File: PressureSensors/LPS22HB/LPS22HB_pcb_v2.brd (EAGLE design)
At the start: 100 x 80 mm, 6 parts

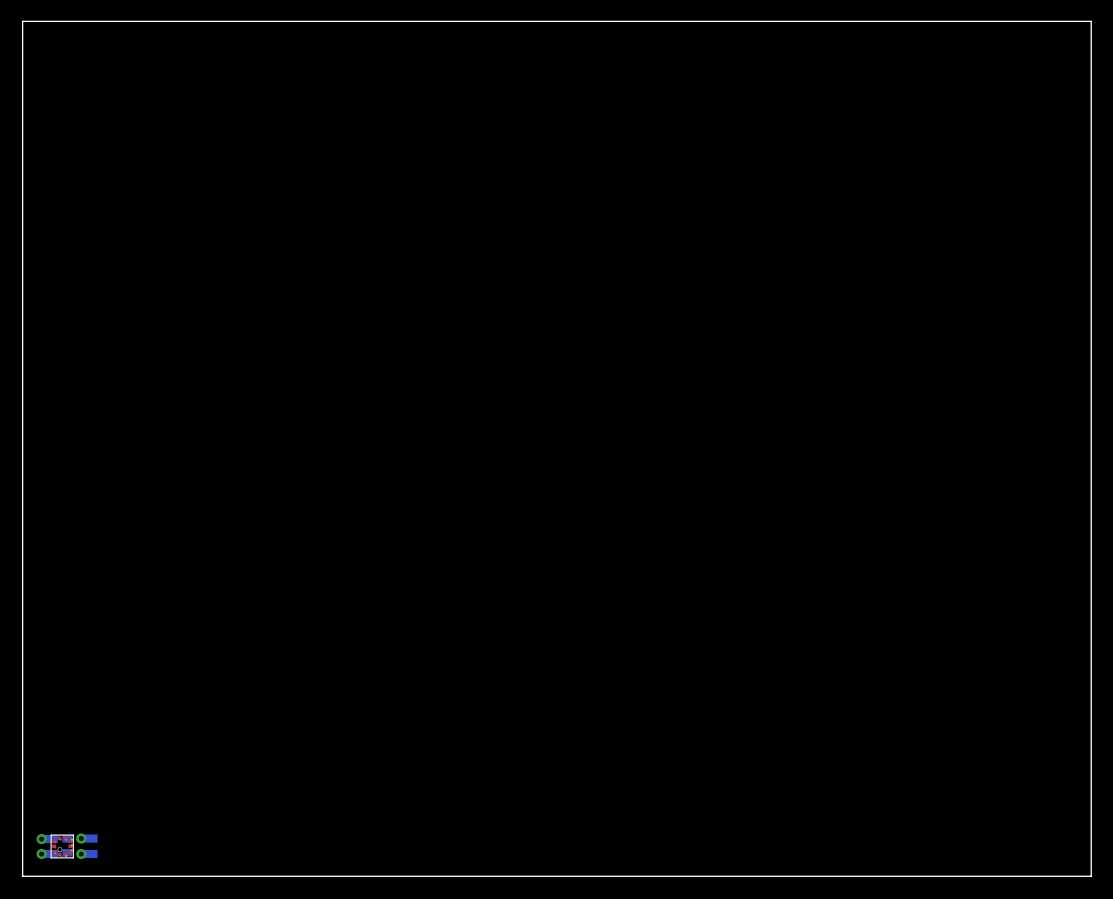
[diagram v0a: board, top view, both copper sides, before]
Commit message: overdue changes before messing with plotPSTHStim
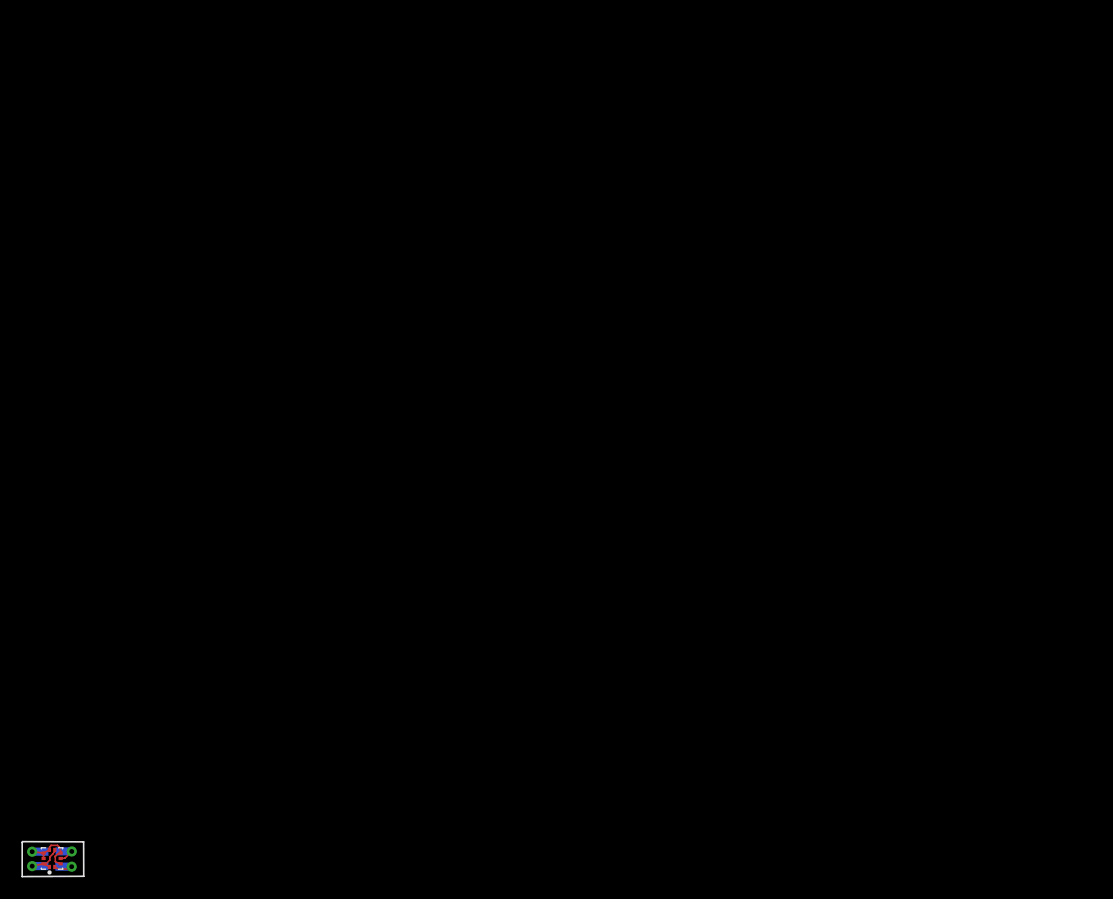
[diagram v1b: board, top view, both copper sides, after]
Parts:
- removed C2: 100nF, resistor:C0402
- removed U$3, U$4, U$5: WIREPAD_PADWIREPAD_0,6/0,4_PAD, Sombeck_lib:WIREPAD_0,6/0,4_PAD
- added U$6, U$7: WIREPAD_PADWIREPAD_0,6/0,4_PAD, Sombeck_lib:WIREPAD_0,6/0,4_PAD
- added U1: LPS22HB, LPS22HB:LGA10R50P2X3_200X200X80
- U$1: value LPS22HB_HLGA -> WIREPAD_PADWIREPAD_0,6/0,4_PAD; device Sombeck_lib:LPS22HB_HLGA -> Sombeck_lib:WIREPAD_0,6/0,4_PAD
- moved U$2 4.60 mm to (0.94, 2.30)
- moved U$1 3.32 mm to (0.94, 0.95), flipped to the bottom
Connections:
- removed net N$1: U$1.P$2, U$2.P$1, U$2.P$2
- removed net N$4: U$1.P$4, U$3.P$1, U$3.P$2
- new net N$2: U$6.P$1, U$6.P$2, U1.2
- new net N$3: U$7.P$1, U$7.P$2, U1.4
- net +3V3: now also U$1.P$2, U1.1, U1.10, U1.6; no longer C2.1, U$1.P$10, U$1.P$6, U$5.P$1, U$5.P$2
- net GND: now also U$2.P$1, U$2.P$2, U1.3, U1.5, U1.7, U1.8, U1.9; no longer C2.2, U$1.P$3, U$1.P$5, U$1.P$7, U$1.P$8, U$1.P$9, U$4.P$1, U$4.P$2
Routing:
- net GND: track 0.00 -> 6.63 mm
- net +3V3: track 0.00 -> 4.52 mm
- net N$2: track 0.00 -> 2.61 mm
- net N$3: track 0.00 -> 2.20 mm
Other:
- board outline removed
